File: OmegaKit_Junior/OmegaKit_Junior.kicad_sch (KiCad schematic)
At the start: 19 parts, among them SW1 SW_CK_OS102011MS2Q, U1 AMS1117-5.0

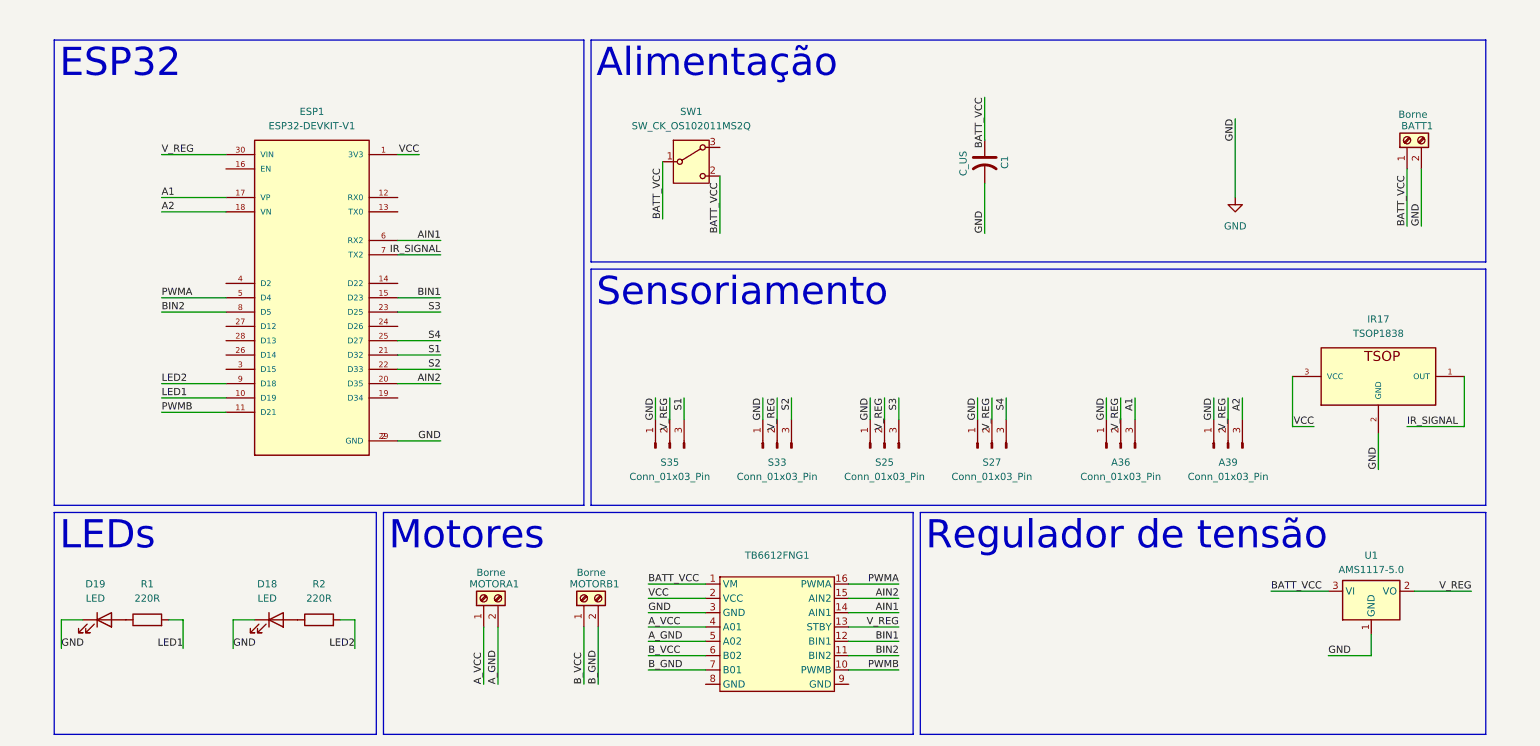
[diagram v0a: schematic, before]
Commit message: Mudanças RZ60 + Placa juniores
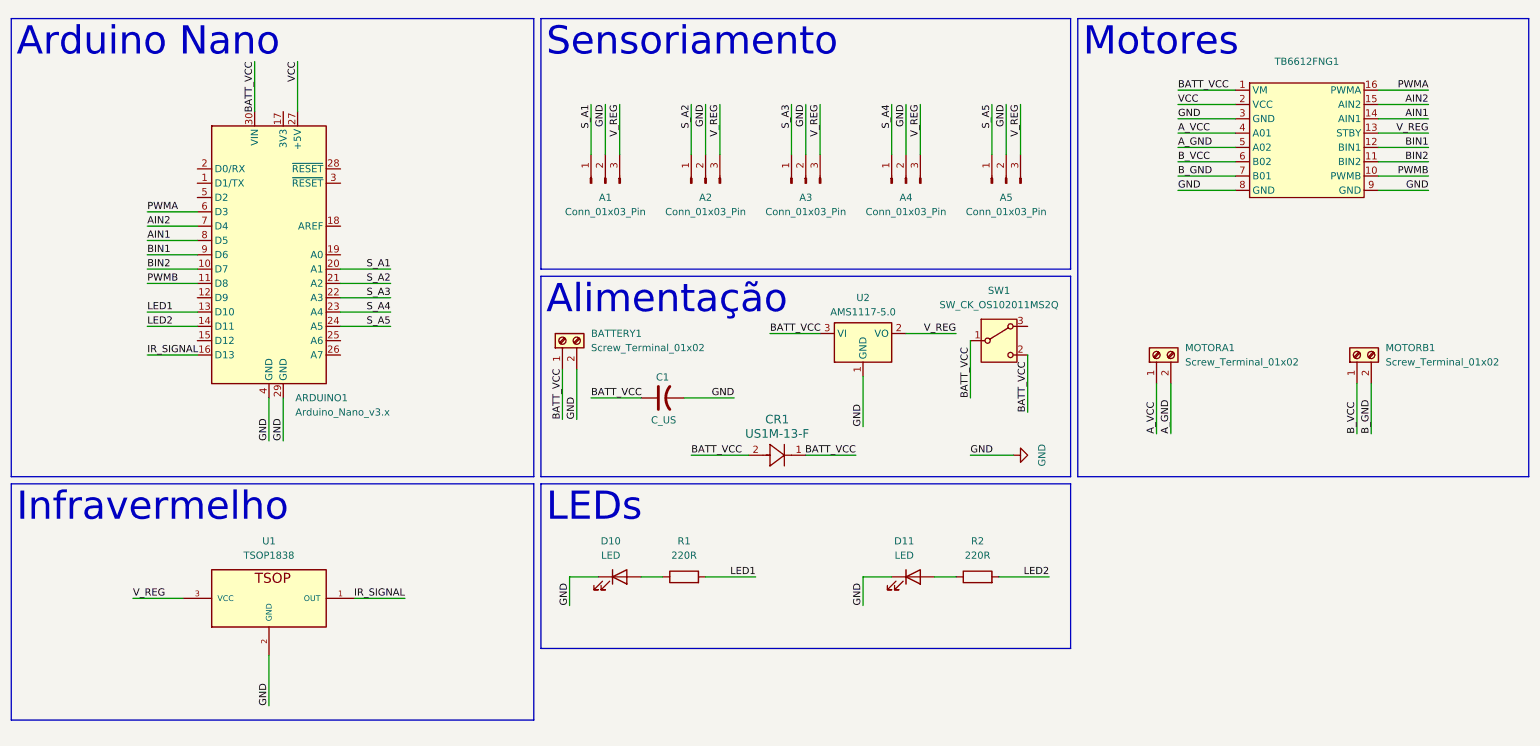
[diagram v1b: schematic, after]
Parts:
- removed A36, A39, S25, S27, S33, S35: Conn_01x03_Pin, Connector_Molex:Molex_KK-254_AE-6410-03A_1x03_P2.54mm_Vertical, symbol Connector:Conn_01x03_Pin
- removed BATT1: Borne, TerminalBlock:TerminalBlock_Xinya_XY308-2.54-2P_1x02_P2.54mm_Horizontal, symbol Connector:Screw_Terminal_01x02
- removed D18, D19: LED, LED_SMD:LED_0805_2012Metric_Pad1.15x1.40mm_HandSolder, symbol Device:LED
- removed ESP1: ESP32-DEVKIT-V1, ESP32-DEVKIT-V1:MODULE_ESP32_DEVKIT_V1, symbol ESP32-DEVKIT-V1:ESP32-DEVKIT-V1
- removed IR17: TSOP1838, TSOP1838:TSOP1838, symbol TSOP1838:TSOP1838
- removed U1: AMS1117-5.0, Package_TO_SOT_SMD:SOT-223-3_TabPin2, symbol Regulator_Linear:AMS1117-5.0
- added A1, A2, A3, A4, A5: Conn_01x03_Pin, Connector_Molex:Molex_KK-254_AE-6410-03A_1x03_P2.54mm_Vertical, symbol Connector:Conn_01x03_Pin
- added ARDUINO1: Arduino_Nano_v3.x, Module:Arduino_Nano, symbol MCU_Module:Arduino_Nano_v3.x
- added BATTERY1: Screw_Terminal_01x02, TerminalBlock:TerminalBlock_Xinya_XY308-2.54-2P_1x02_P2.54mm_Horizontal, symbol Connector:Screw_Terminal_01x02
- added CR1: US1M-13-F, SMA_DIO, symbol 2025-08-08_11-05-47:US1M-13-F
- added D10, D11: LED, LED_SMD:LED_0805_2012Metric_Pad1.15x1.40mm_HandSolder, symbol Device:LED
- added U1: TSOP1838, TSOP1838:TSOP1838, symbol TSOP1838:TSOP1838
- added U2: AMS1117-5.0, Package_TO_SOT_SMD:SOT-223-3_TabPin2, symbol Regulator_Linear:AMS1117-5.0
- C1: footprint Capacitor_THT:C_Radial_D5.0mm_H5.0mm_P2.00mm -> Capacitor_THT:C_Radial_D4.0mm_H5.0mm_P1.50mm
- MOTORA1, MOTORB1: value Borne -> Screw_Terminal_01x02
- R1, R2: footprint Resistor_SMD:R_0805_2012Metric_Pad1.20x1.40mm_HandSolder -> Resistor_SMD:R_0805_2012Metric
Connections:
- net AIN1: now also ARDUINO1.8 (D5)
- net AIN2: now also ARDUINO1.7 (D4)
- net BATT_VCC: now also ARDUINO1.30 (VIN), BATTERY1.1 (Pin_1), CR1.1, CR1.2, U2.3 (VI)
- net BIN1: now also ARDUINO1.9 (D6)
- net BIN2: now also ARDUINO1.10 (D7)
- net GND: now also TB6612FNG1.8 (GND), TB6612FNG1.9 (GND), A1.2 (Pin_2), A2.2 (Pin_2), A3.2 (Pin_2), A4.2 (Pin_2), A5.2 (Pin_2), ARDUINO1.29 (GND), ARDUINO1.4 (GND), BATTERY1.2 (Pin_2), D10.1 (K), D11.1 (K), U1.2 (GND), U2.1 (GND)
- net IR_SIGNAL: now also ARDUINO1.16 (D13), U1.1 (OUT)
- net LED1: now also ARDUINO1.13 (D10)
- net LED2: now also ARDUINO1.14 (D11)
- net PWMA: now also ARDUINO1.6 (D3)
- net PWMB: now also ARDUINO1.11 (D8)
- net VCC: now also ARDUINO1.27 (+5V)
- net V_REG: now also A1.3 (Pin_3), A2.3 (Pin_3), A3.3 (Pin_3), A4.3 (Pin_3), A5.3 (Pin_3), U1.3 (VCC), U2.2 (VO)
- net at R2.1: now also D11.2 (A)
- net at R1.1: now also D10.2 (A)
- new net S_A1: A1.1 (Pin_1), ARDUINO1.20 (A1)
- new net S_A2: A2.1 (Pin_1), ARDUINO1.21 (A2)
- new net S_A3: A3.1 (Pin_1), ARDUINO1.22 (A3)
- new net S_A4: A4.1 (Pin_1), ARDUINO1.23 (A4)
- new net S_A5: A5.1 (Pin_1), ARDUINO1.24 (A5)
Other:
- moved on the sheet: SW1
